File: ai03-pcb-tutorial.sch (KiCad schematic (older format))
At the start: 24 parts, among them SW1 SW_PUSH, U1 ATmega32U4-AU, Y1 16MHz

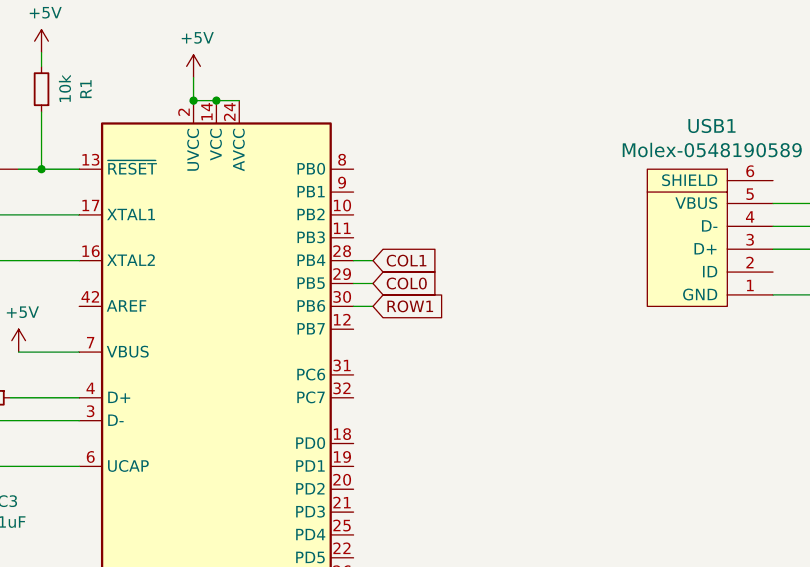
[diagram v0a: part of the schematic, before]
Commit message: adjust routeing
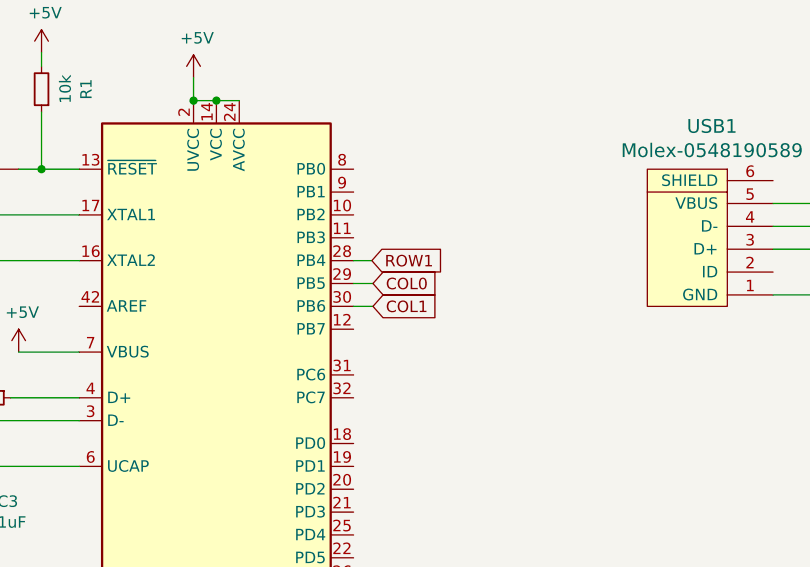
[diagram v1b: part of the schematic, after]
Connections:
- net COL1: now also U1.30 (PB6); no longer U1.28 (PB4)
- net ROW1: now also U1.28 (PB4); no longer U1.30 (PB6)
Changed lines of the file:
@@
 Wire Wire Line
 	5550 2100 5900 2100
-Text GLabel 3800 2350 2    50   Input ~ 0
-COL0
 Text GLabel 3765 3750 2    50   Input ~ 0
 ROW0
-Text GLabel 3800 2450 2    50   Input ~ 0
-ROW1
-Text GLabel 3800 2250 2    50   Input ~ 0
-COL1
-Wire Wire Line
-	3715 2250 3800 2250
-Wire Wire Line
-	3800 2350 3715 2350
 Wire Wire Line
 	3715 2450 3800 2450
@@
 	5550 2000 5805 2000
 Connection ~ 5805 2000
+Wire Wire Line
+	3795 2250 3715 2250
+Wire Wire Line
+	3800 2350 3715 2350
+Text GLabel 3800 2350 2    50   Input ~ 0
+COL0
+Text GLabel 3800 2450 2    50   Input ~ 0
+COL1
+Text GLabel 3795 2250 2    50   Input ~ 0
+ROW1
 $EndSCHEMATC
